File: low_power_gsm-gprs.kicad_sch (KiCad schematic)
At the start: 38 parts, among them J1 Conn_Coaxial, J2 SIM_Card, J3 Conn_02x20_Odd_Even, J4 USB_B_Micro, Q1 2N7002, Q2 2N7002, U1 SARA-G450, U2 PL2303SA, U3 LT1764AEQ#PBF

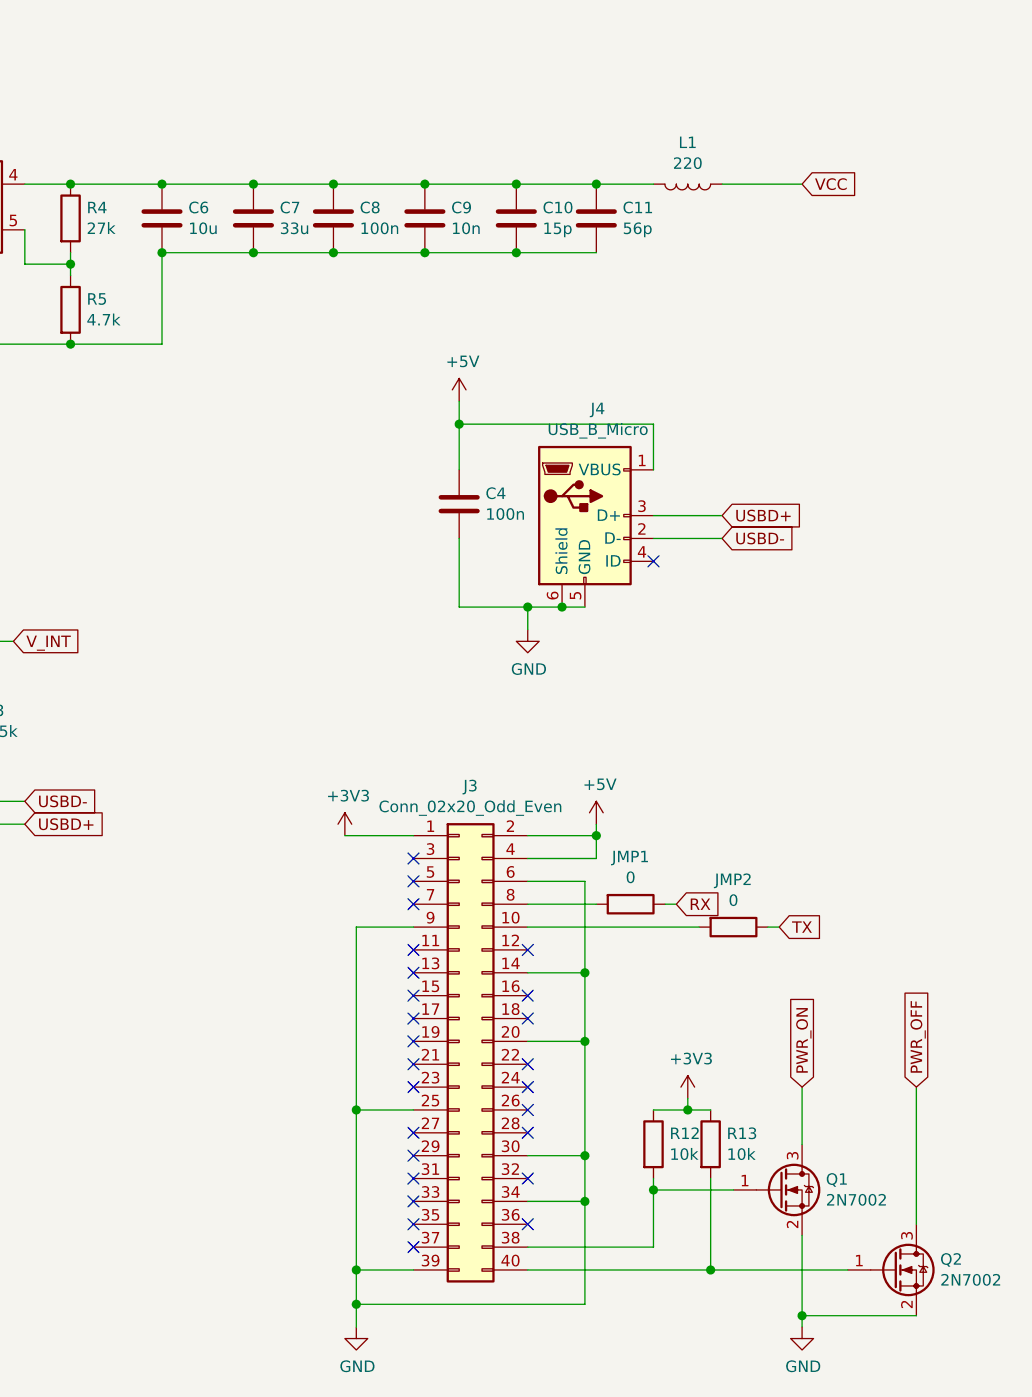
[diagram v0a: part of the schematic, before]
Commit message: Updated board power supply
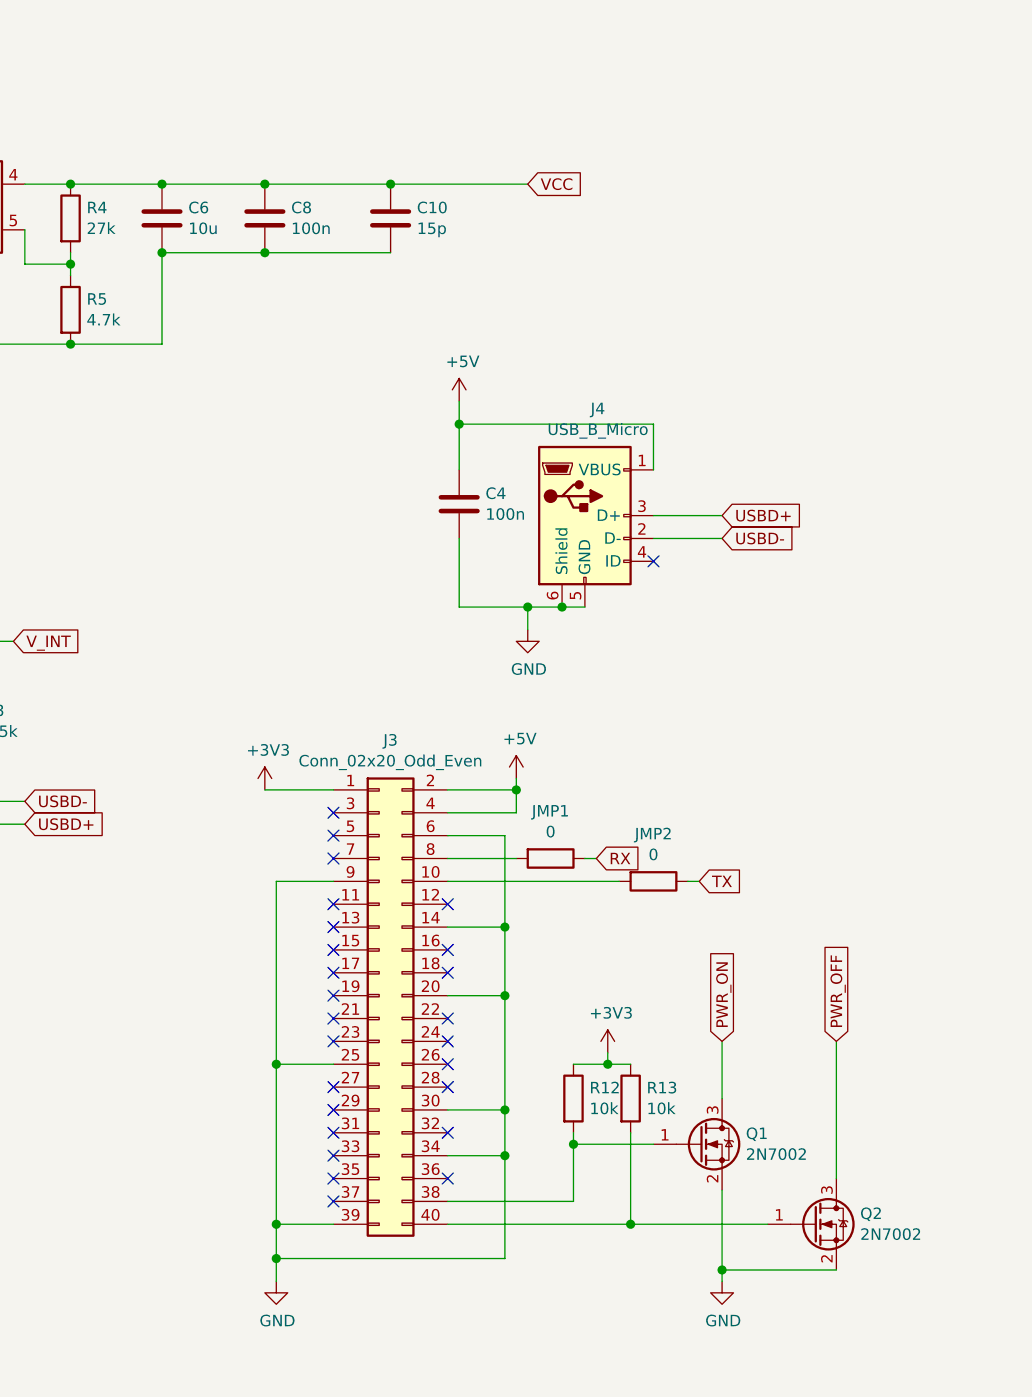
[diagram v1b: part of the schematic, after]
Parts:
- removed C11: 56p, Capacitor_SMD:C_0805_2012Metric, symbol Device:C
- removed C7: 33u, Capacitor_SMD:C_0805_2012Metric, symbol Device:C
- removed C9: 10n, Capacitor_SMD:C_0805_2012Metric, symbol Device:C
- removed L1: 220, Inductor_SMD:L_0805_2012Metric, symbol Device:L
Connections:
- net VCC: now also C10.1, C6.1, C8.1, R4.1, U3.4 (OUT)
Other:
- moved on the sheet: C10, C8, J3, JMP1, JMP2, Q1, Q2, R12, R13
